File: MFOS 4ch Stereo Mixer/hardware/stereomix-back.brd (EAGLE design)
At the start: 30.1 x 113 mm, 27 parts, among them IC1 TL082P

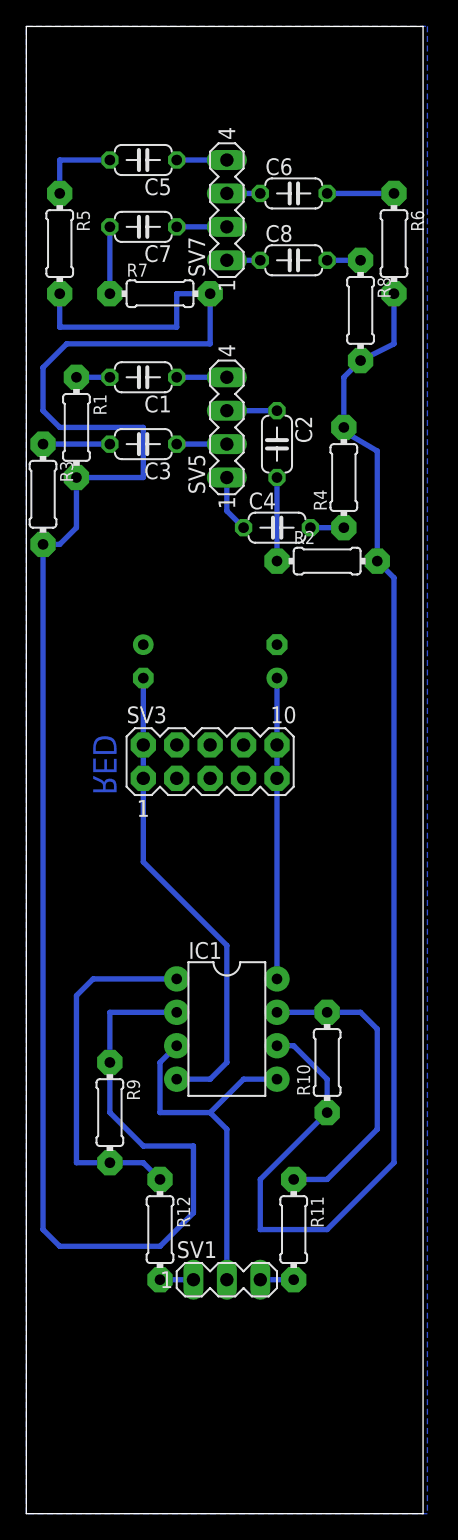
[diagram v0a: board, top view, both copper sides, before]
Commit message: Add files via upload
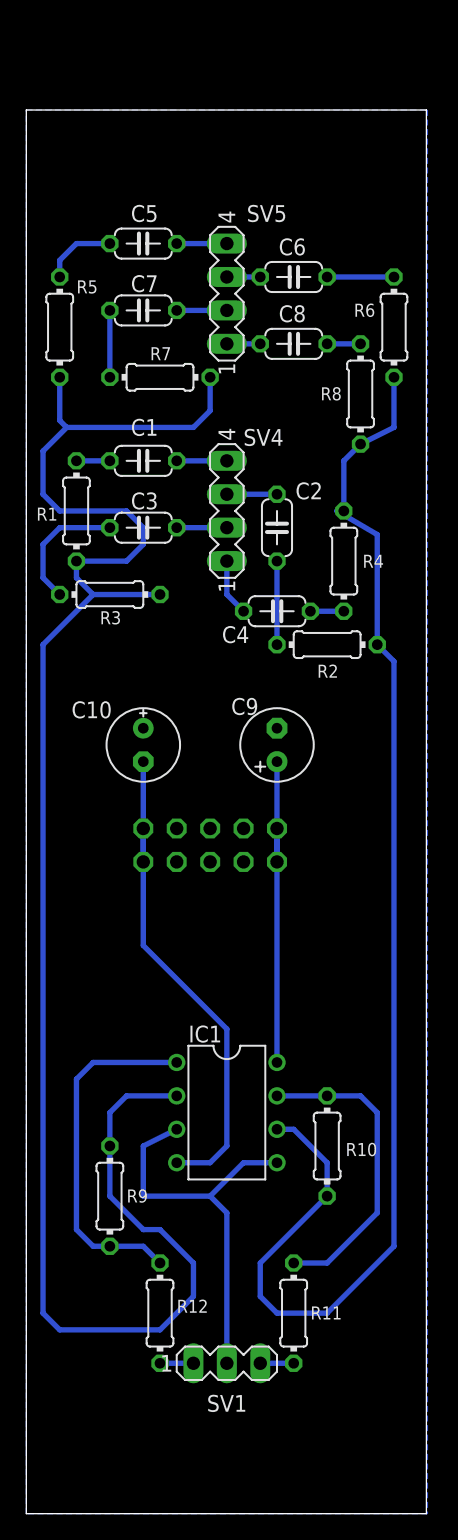
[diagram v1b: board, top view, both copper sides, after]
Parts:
- removed SV7: (no value), con-lstb:MA04-1
- added SV4: (no value), con-lstb:MA04-1
- C10, C9: value (none) -> 100µ
- moved SV5 10.2 mm to (15.2, 92.7)
- moved R3 9.16 mm to (6.35, 69.8), turned to 0 degrees
- moved C4 6.35 mm to (19.1, 68.6)
- moved C5 6.35 mm to (8.89, 96.5)
- moved C7 6.35 mm to (8.89, 91.4)
- moved R9 6.35 mm to (6.35, 24.1)
- moved SV1 6.35 mm to (15.2, 11.4)
- moved SV3 6.35 mm to (14.0, 50.8), flipped to the bottom, turned to 180 degrees
- moved R11 6.35 mm to (20.3, 15.2)
- moved R12 6.35 mm to (10.2, 15.2)
- moved IC1 6.35 mm to (15.2, 30.5)
- moved R10 6.35 mm to (22.9, 27.9)
- moved C1 6.35 mm to (8.89, 80.0)
- moved C10 6.35 mm to (8.89, 58.4), flipped to the top
- moved C2 6.35 mm to (19.1, 74.9)
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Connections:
- net N$35: now also SV5.1; no longer SV7.1
- net N$36: now also SV5.2; no longer SV7.2
- net N$37: now also SV5.3; no longer SV7.3
- net N$38: now also SV5.4; no longer SV7.4
- net N$39: now also SV4.1; no longer SV5.1
- net N$40: now also SV4.2; no longer SV5.2
- net N$41: now also SV4.3; no longer SV5.3
- net N$42: now also SV4.4; no longer SV5.4
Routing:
- net N$1: track 151.2 -> 139.7 mm
- net N$8: track 5.08 -> 9.94 mm
- net N$16: track 36.2 -> 38.7 mm
- net N$15: track 22.9 -> 25.4 mm
- net GND2: track 28.8 -> 31.1 mm
- net N$10: track 6.35 -> 5.61 mm
- net N$2: track 27.7 -> 27.0 mm
- net N$4: track 101.6 -> 100.9 mm
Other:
- board size 30.1 x 113 mm -> 30.4 x 106.7 mm
